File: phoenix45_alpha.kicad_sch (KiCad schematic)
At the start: 125 parts, among them J1 AVR-ISP-6, SW1 SW_PUSH, SW2 SW_PUSH, U1 SRV05-4, U2 ATmega32U4-M, U3 ATmega32U4-M, X1 Crystal_GND24_Small

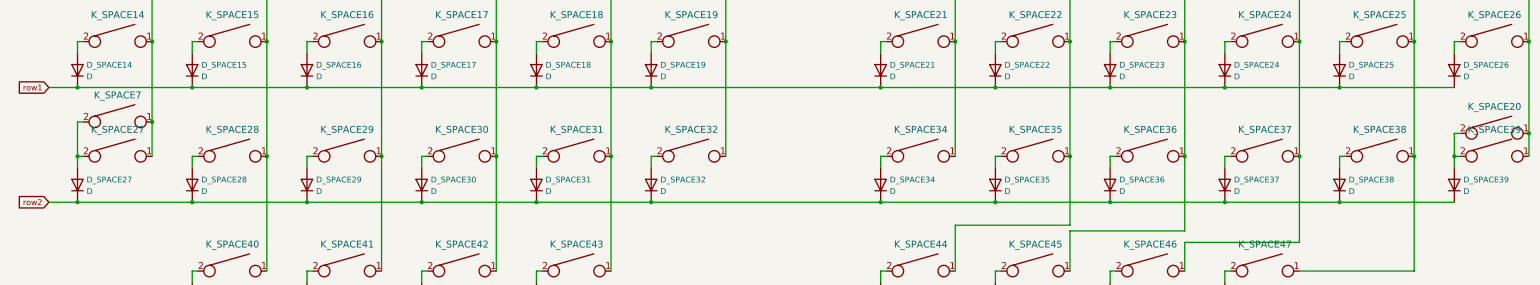
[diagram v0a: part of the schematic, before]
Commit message: MX+choc
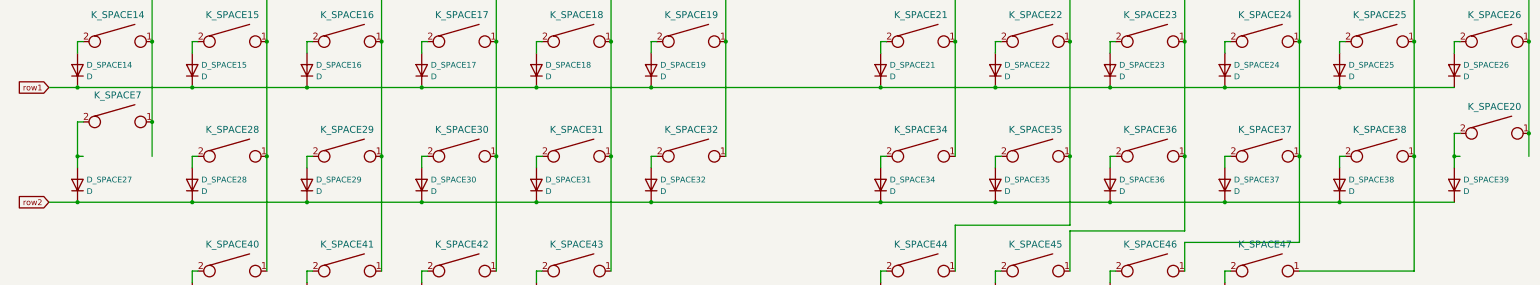
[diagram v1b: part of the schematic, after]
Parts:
- removed K_SPACE27, K_SPACE39: KEYSW, MX_Only:MXOnly-1U-NoLED, symbol keyboard_parts:KEYSW
- K_SPACE1, K_SPACE10, K_SPACE11, K_SPACE12, K_SPACE13, K_SPACE14, K_SPACE15, K_SPACE16, K_SPACE17, K_SPACE18, K_SPACE19, K_SPACE2, K_SPACE21, K_SPACE22, K_SPACE23, K_SPACE24, K_SPACE25, K_SPACE26, K_SPACE28, K_SPACE29, K_SPACE3, K_SPACE30, K_SPACE31, K_SPACE32, K_SPACE34, K_SPACE35, K_SPACE36, K_SPACE37, K_SPACE38, K_SPACE4, K_SPACE41, K_SPACE46, K_SPACE5, K_SPACE6, K_SPACE8, K_SPACE9: footprint MX_Only:MXOnly-1U-NoLED -> kbd:CherryMX_Choc_1u
- K_SPACE20, K_SPACE7: footprint MX_Only:MXOnly-1.5U-NoLED -> kbd:CherryMX_Choc_1.5u
- K_SPACE40, K_SPACE47: footprint MX_Only:MXOnly-1.25U-NoLED -> kbd:CherryMX_Choc_1.5u
- K_SPACE42, K_SPACE45: footprint MX_Only:MXOnly-1.25U-NoLED -> kbd:CherryMX_Choc_1u
- K_SPACE43, K_SPACE44: footprint MX_Only:MXOnly-1.75U-NoLED -> kbd:CherryMX_Choc_1.5u

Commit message: go back to MX
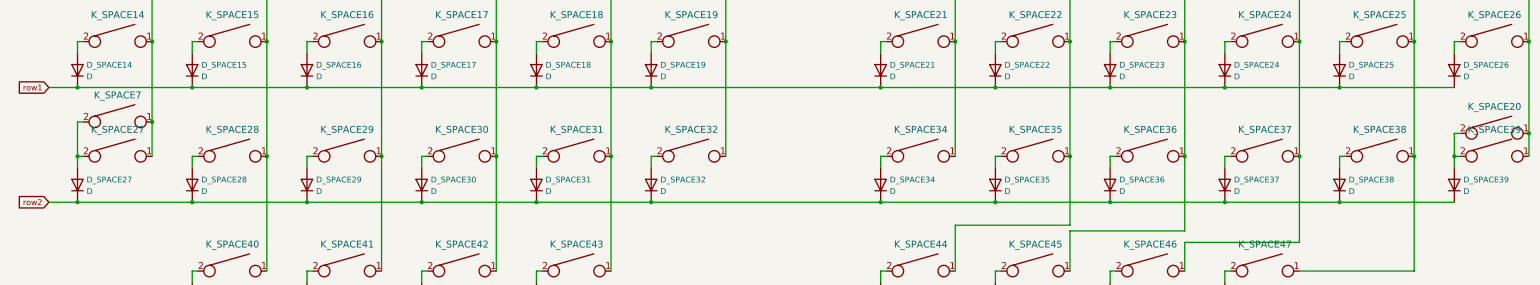
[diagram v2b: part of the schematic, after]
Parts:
- added K_SPACE27, K_SPACE39: KEYSW, MX_Only:MXOnly-1U-NoLED, symbol keyboard_parts:KEYSW
- K_SPACE1, K_SPACE10, K_SPACE11, K_SPACE12, K_SPACE13, K_SPACE14, K_SPACE15, K_SPACE16, K_SPACE17, K_SPACE18, K_SPACE19, K_SPACE2, K_SPACE21, K_SPACE22, K_SPACE23, K_SPACE24, K_SPACE25, K_SPACE26, K_SPACE28, K_SPACE29, K_SPACE3, K_SPACE30, K_SPACE31, K_SPACE32, K_SPACE34, K_SPACE35, K_SPACE36, K_SPACE37, K_SPACE38, K_SPACE4, K_SPACE41, K_SPACE46, K_SPACE5, K_SPACE6, K_SPACE8, K_SPACE9: footprint kbd:CherryMX_Choc_1u -> MX_Only:MXOnly-1U-NoLED
- K_SPACE20, K_SPACE7: footprint kbd:CherryMX_Choc_1.5u -> MX_Only:MXOnly-1.5U-NoLED
- K_SPACE40, K_SPACE47: footprint kbd:CherryMX_Choc_1.5u -> MX_Only:MXOnly-1.25U-NoLED
- K_SPACE42, K_SPACE45: footprint kbd:CherryMX_Choc_1u -> MX_Only:MXOnly-1.25U-NoLED
- K_SPACE43, K_SPACE44: footprint kbd:CherryMX_Choc_1.5u -> MX_Only:MXOnly-1.75U-NoLED
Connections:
- net col0: now also K_SPACE27.1
- net col12: now also K_SPACE39.1
- net at D_SPACE39.2 (A), K_SPACE20.2: now also K_SPACE39.2
- net at D_SPACE27.2 (A), K_SPACE7.2: now also K_SPACE27.2
